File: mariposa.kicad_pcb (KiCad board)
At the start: 2 copper layers, 52.1 x 109 mm, 53 parts, among them J1 Conn_01x22_Shielded, J2 Conn_01x03_MountingPin, J3 Conn_ARM_SWD_TagConnect_TC203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, J4 USB_C_Receptacle_USB2.0_16P, J5 Conn_02x03_Counter_Clockwise, J6 Conn_01x05_Socket, SW1 SW_Push, SW2 Slide_DPDT_SS22D06, SW3 SW_Push, U2 TPS7A0333PDBVR, U3 MCP73831T-2ACI/OT

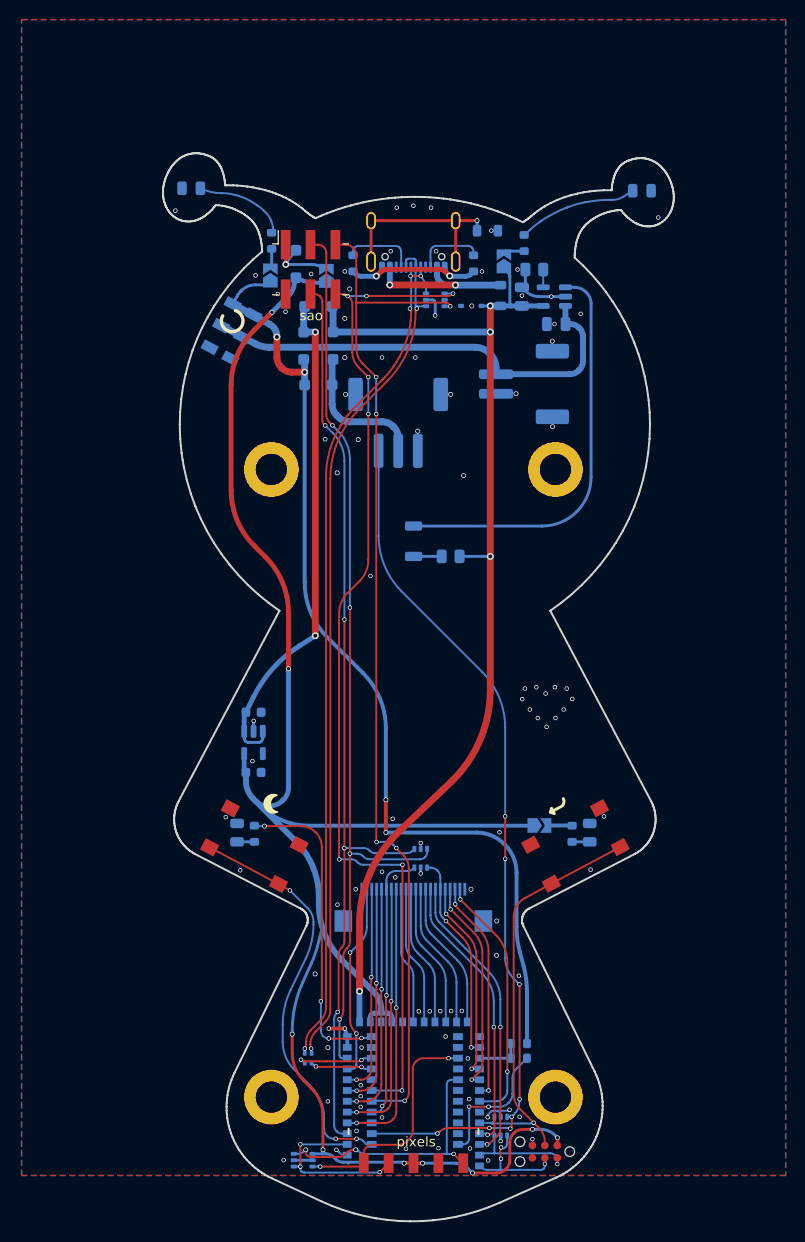
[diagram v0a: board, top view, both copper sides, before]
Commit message: mariposa v2 RC2
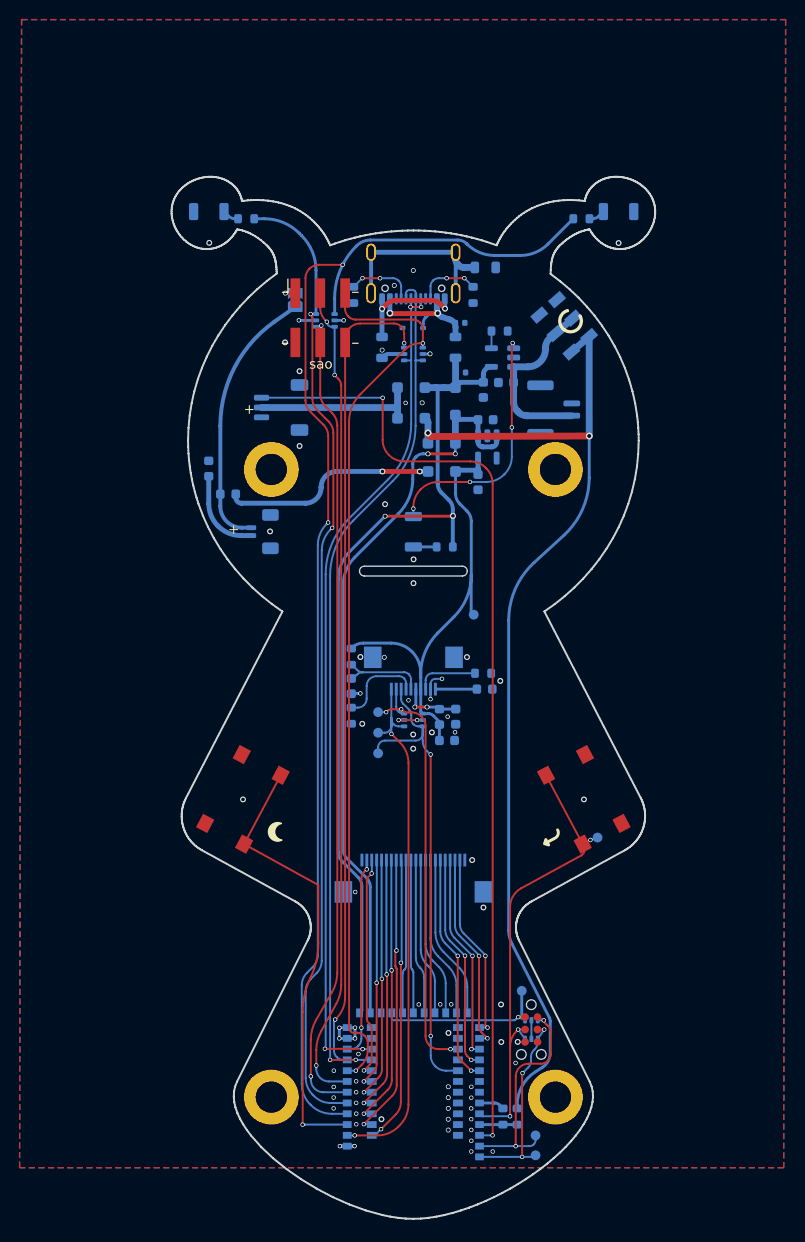
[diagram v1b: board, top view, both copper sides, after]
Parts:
- removed D7, D8: LED, LED_SMD:LED_0805_2012Metric
- removed JP2, JP3, JP4: SolderJumper_2_Open, Jumper:SolderJumper-2_P1.3mm_Open_TrianglePad1.0x1.5mm
- removed R11: 20k, Resistor_SMD:R_0603_1608Metric
- removed R12: 12k, Resistor_SMD:R_0603_1608Metric
- removed RN1: 2x R22, PCM_Resistor_SMD_AKL:R_Array_Convex_2x0402
- added C1: 560pF, Capacitor_SMD:C_0603_1608Metric, B.Cu at (143.7, 88.0)
- added C2: 1uF, Capacitor_SMD:C_0603_1608Metric, B.Cu at (154.3, 91.2)
- added C3: 1uF, Capacitor_SMD:C_0603_1608Metric, B.Cu at (153.4, 93.6)
- added C4: 10nF, Capacitor_SMD:C_0402_1005Metric, B.Cu at (154.8, 51.0)
- added C5: 10nF, Capacitor_SMD:C_0402_1005Metric, B.Cu at (154.8, 56.0)
- added FB3: 240 Ohm, PCM_Ferrite_SMD_AKL:Ferrite_0603_1608Metric, B.Cu at (152.7, 91.2)
- added FB4: 240 Ohm, PCM_Ferrite_SMD_AKL:Ferrite_0603_1608Metric, B.Cu at (157.3, 88.3)
- added FB5: 120 Ohm, PCM_Ferrite_SMD_AKL:Ferrite_0805_2012Metric, B.Cu at (146.8, 53.5)
- added FB6: 240 Ohm, PCM_Ferrite_SMD_AKL:Ferrite_0603_1608Metric, B.Cu at (131.1, 68.4)
- added FB7: 240 Ohm, PCM_Ferrite_SMD_AKL:Ferrite_0603_1608Metric, B.Cu at (129.1, 65.8)
- added J7: Ext VCC Out, Connector_JST:JST_SUR_SM02B-SURS-TF_1x02-1MP_P0.80mm_Horizontal, B.Cu at (134.6, 72.3)
- added R13: 10k, Resistor_SMD:R_0603_1608Metric, B.Cu at (157.1, 86.7)
- added R5: 10k, Resistor_SMD:R_0603_1608Metric, B.Cu at (143.7, 91.1)
- added R6: 10k, Resistor_SMD:R_0603_1608Metric, B.Cu at (143.7, 85.0)
- added TP1: TestPoint, TestPoint:TestPoint_Pad_D1.0mm, B.Cu at (162.5, 135.9)
- added TP2: TestPoint, TestPoint:TestPoint_Pad_D1.0mm, B.Cu at (162.5, 133.9)
- added TP3: TestPoint, TestPoint:TestPoint_Pad_D1.0mm, B.Cu at (168.8, 103.5)
- added TP4: TestPoint, TestPoint:TestPoint_Pad_D1.0mm, B.Cu at (156.2, 80.8)
- added TP5: TestPoint, TestPoint:TestPoint_Pad_D1.0mm, B.Cu at (161.1, 119.2)
- added TP6: TestPoint, TestPoint:TestPoint_Pad_D1.0mm, B.Cu at (146.4, 92.8)
- added TP7: TestPoint, TestPoint:TestPoint_Pad_D1.0mm, B.Cu at (146.4, 90.7)
- added TP8: TestPoint, TestPoint:TestPoint_Pad_D1.0mm, B.Cu at (146.4, 94.9)
- BT1: footprint Connector_JST:JST_PH_S2B-PH-SM4-TB_1x02-1MP_P2.00mm_Horizontal -> Connector_JST:JST_GH_SM02B-GHS-TB_1x02-1MP_P1.25mm_Horizontal
- C46, C47: footprint Capacitor_SMD:C_0805_2012Metric -> Capacitor_SMD:C_0603_1608Metric
- D5, D6: footprint LED_SMD:LED_0805_2012Metric -> LED_SMD:LED_1206_3216Metric_ReverseMount_Hole1.8x2.4mm
- FB1, FB2: value 60ohm -> 120 Ohm
- J2: footprint Connector_JST:JST_PH_S3B-PH-SM4-TB_1x03-1MP_P2.00mm_Horizontal -> Connector_JST:JST_SH_SM03B-SRSS-TB_1x03-1MP_P1.00mm_Horizontal
- J6: value Conn_01x05_Socket -> Conn_01x10_MountingPin; footprint coquette_footprints:5-pin horizontal display -> Connector_FFC-FPC:Hirose_FH12-10S-0.5SH_1x10-1MP_P0.50mm_Horizontal; moved to B.Cu
- R1, R8: footprint Resistor_SMD:R_0805_2012Metric -> Resistor_SMD:R_0603_1608Metric
- R2, R7: value 3k -> 2k
- moved D6 74.4 mm to (170.9, 39.6), turned to 180 degrees
- moved D5 74.4 mm to (129.1, 39.6), turned to 0 degrees
- moved R7 71.1 mm to (167.2, 40.3), turned to 180 degrees
- moved R2 71.1 mm to (132.9, 40.3), turned to 0 degrees
- moved D12 55.8 mm to (141.0, 50.7), turned to 180 degrees
- moved D11 46.3 mm to (150.0, 91.5)
- moved J6 45.0 mm to (150.0, 86.5)
- moved U2 38.5 mm to (157.6, 63.6)
- moved C44 38.1 mm to (157.4, 60.9)
- moved C45 37.5 mm to (156.6, 67.2), turned to -90 degrees
- moved SW2 34.0 mm to (165.4, 51.3), turned to -49 degrees
- moved D4 25.9 mm to (152.9, 66.1), turned to 0 degrees
- moved D45 17.2 mm to (152.9, 63.2), turned to 180 degrees
- moved D88 17.0 mm to (154.3, 59.0), turned to 90 degrees
- moved J3 12.5 mm to (162.0, 123.1), turned to -90 degrees
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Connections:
- net row_e renamed ch5
- C44 pad 1: Net-(D45-K) -> VDC
- D10 pad 1: /power/IN_D- -> gpio1
- D10 pad 3: /power/IN_D+ -> D-
- D10 pad 4: gpio2 -> D+
- D10 pad 6: gpio1 -> gpio2
- D11 pad 3: mosi -> cs
- D11 pad 6: cs -> mosi
- D12 pad 1: gpio4 -> status_led_2
- D12 pad 3: gpio3 -> sda
- D12 pad 6: sda -> status_led_1
- D13 pad 1: swdclk -> VDD
- D13 pad 4: reset -> swdclk
- D13 pad 6: led_data -> reset
- D45 pad 1: Net-(D45-K) -> VDC
- D88 pad 1: Net-(D45-K) -> VDC
- D9 pad 2: VBUS -> Net-(C4--)
- FB1 pad 1: Net-(FB1-Pad1) -> Net-(C4--)
- J1 pad 10: c4 -> ch10
- J1 pad 11: c3 -> ch11
- J1 pad 12: c2 -> ch12
- J1 pad 13: c1 -> ch13
- J1 pad 14: c0 -> ch14
- J1 pad 15: ec1b -> ch15
- J1 pad 16: ec1a -> ch16
- J1 pad 17: gpio3 -> ch17
- J1 pad 18: row_d -> ch18
- J1 pad 19: row_c -> ch19
- J1 pad 2: row_h -> ch2
- J1 pad 20: row_b -> ch20
- J1 pad 21: row_a -> ch21
- J1 pad 3: row_g -> ch3
- J1 pad 4: row_f -> ch4
- J1 pad 6: gpio4 -> ch6
- J1 pad 7: ec2b -> ch7
- J1 pad 8: ec2a -> ch8
- J1 pad 9: c5 -> ch9
- J3 pad 1: VCC -> VDD
- J4 pad A1: GND -> Net-(FB5-Pad2)
- J4 pad A12: GND -> Net-(FB5-Pad2)
- J4 pad A4: Net-(FB1-Pad1) -> Net-(C4--)
- J4 pad A6: /power/IN_D+ -> D+
- J4 pad A7: /power/IN_D- -> D-
- J4 pad A9: Net-(FB1-Pad1) -> Net-(C4--)
- J4 pad B1: GND -> Net-(FB5-Pad2)
- J4 pad B12: GND -> Net-(FB5-Pad2)
- J4 pad B4: Net-(FB1-Pad1) -> Net-(C4--)
- J4 pad B6: /power/IN_D+ -> D+
- J4 pad B7: /power/IN_D- -> D-
- J4 pad B9: Net-(FB1-Pad1) -> Net-(C4--)
- J5 pad 1: Net-(D4-K) -> Net-(J5-Pin_1)
- J6 pad 1: mosi -> sck
- J6 pad 2: sck -> mosi
- J6 pad 3: VCC -> cs
- J6 pad 4: GND -> Net-(J6-Pin_4)
- J6 pad 5: cs -> Net-(J6-Pin_5)
- JP1 pad 1: VCC -> PRI_MID
- JP1 pad 2: Net-(D4-K) -> Net-(J5-Pin_1)
- R2 pad 2: Net-(JP4-B) -> status_led_1
- R7 pad 2: status_led -> status_led_2
- SW1 pad 2: Net-(U1-P0.30) -> Net-(U1-P1.03)
- U1 pad 10: sda -> ch21
- U1 pad 14: VCC -> VDC
- U1 pad 16: VCC -> VDD
- U1 pad 17: unconnected-(U1-P0.13-Pad17) -> ch13
- U1 pad 18: c0 -> ch12
- U1 pad 19: c1 -> ch11
- U1 pad 20: c2 -> ch10
- U1 pad 21: c3 -> ch9
- U1 pad 22: c4 -> ch8
- U1 pad 23: c5 -> ch7
- U1 pad 24: unconnected-(U1-P1.07-Pad24) -> ch2
- U1 pad 25: gpio4 -> ch3
- U1 pad 26: BATT_READ -> ch4
- U1 pad 28: row_f -> ch6
- U1 pad 29: row_g -> unconnected-(U1-P0.21-Pad29)
- U1 pad 3: scl -> Net-(U1-P1.03)
- U1 pad 30: row_h -> unconnected-(U1-P1.06-Pad30)
- U1 pad 31: unconnected-(U1-P0.27-Pad31) -> BATT_READ_EN
- U1 pad 33: ec2a -> BATT_READ
- U1 pad 34: ec2b -> led_data
- U1 pad 37: Net-(U1-P0.30) -> ch14
- U1 pad 38: led_data -> ch15
- U1 pad 39: unconnected-(U1-P1.11-Pad39) -> ch16
- U1 pad 4: ec1b -> status_led_2
- U1 pad 40: gpio3 -> ch17
- U1 pad 41: gpio1 -> ch18
- U1 pad 42: gpio2 -> ch19
- U1 pad 43: unconnected-(U1-P1.15-Pad43) -> ch20
- U1 pad 47: status_led -> unconnected-(U1-P0.03-Pad47)
- U1 pad 5: ec1a -> status_led_1
- U1 pad 58: BATT_READ_EN -> unconnected-(U1-P0.26-Pad58)
- U1 pad 6: row_d -> scl
- U1 pad 7: row_c -> sda
- U1 pad 8: row_b -> gpio1
- U1 pad 9: row_a -> gpio2
- U2 pad 1: Net-(D45-K) -> VDC
- U2 pad 3: Net-(D45-K) -> VDC
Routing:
- net VCC: track 181.6 -> 48.2 mm, vias 9 -> 0
- net status_led_2: track 0.00 -> 126.3 mm, vias 0 -> 2
- net status_led_1: track 0.00 -> 99.5 mm, vias 0 -> 2
- net /power/IN_D+: track 87.6 -> 0.00 mm, vias 4 -> 0
- net /power/IN_D-: track 87.2 -> 0.00 mm, vias 2 -> 0
- net D-: track 6.36 -> 88.0 mm
- net D+: track 7.90 -> 86.9 mm, vias 2 -> 4
- net VDC: track 0.00 -> 76.3 mm, vias 0 -> 2
- net Net-(D45-K): track 51.0 -> 0.00 mm, vias 2 -> 0
- net Net-(U1-P1.03): track 0.00 -> 45.9 mm, vias 0 -> 1
- net Net-(U1-P0.30): track 41.7 -> 0.00 mm, vias 3 -> 0
- net sck: track 17.6 -> 56.0 mm, vias 3 -> 2
- net status_led: track 32.4 -> 0.00 mm, vias 4 -> 0
- net ec2b: track 29.9 -> 0.00 mm, vias 2 -> 0
- net ch14: track 0.00 -> 29.2 mm, vias 0 -> 2
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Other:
- board size 52.1 x 109 mm -> 49.4 x 106.4 mm
- board text added: "+"
- board text added: "10nF"
- board text added: "2"
- board text added: "2k"
- board text added: "3"
- board text added: "3.3v reg"
- board text added: "battery pwr"
- board text added: "reset"
- board text added: "sao pwr"
- board text added: "swdclk"
- board text added: "swdio"
- board text removed: "22"
- board text removed: "3k"
- board text removed: "VCC reg"
- board text removed: "bat pwr"
- board text removed: "by"
- board text removed: "sao power"
- board text removed: "status"
- board text removed: "vbus"
- board text removed: "vcc"
